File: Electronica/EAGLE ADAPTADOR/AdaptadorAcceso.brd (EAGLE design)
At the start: 160.5 x 111 mm, 9 parts

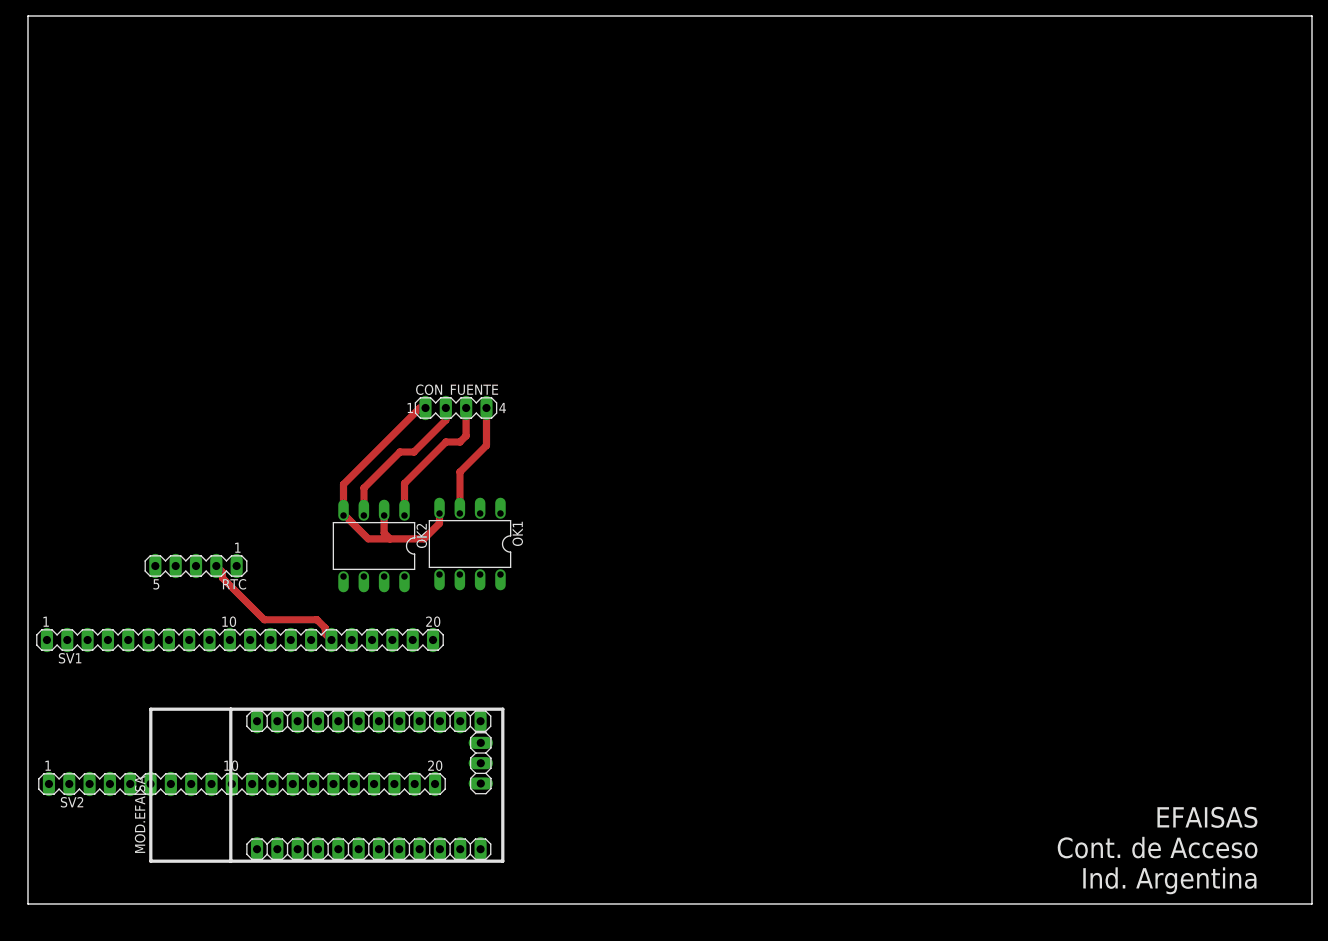
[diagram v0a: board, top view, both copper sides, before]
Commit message: PCB terminado - A revisar
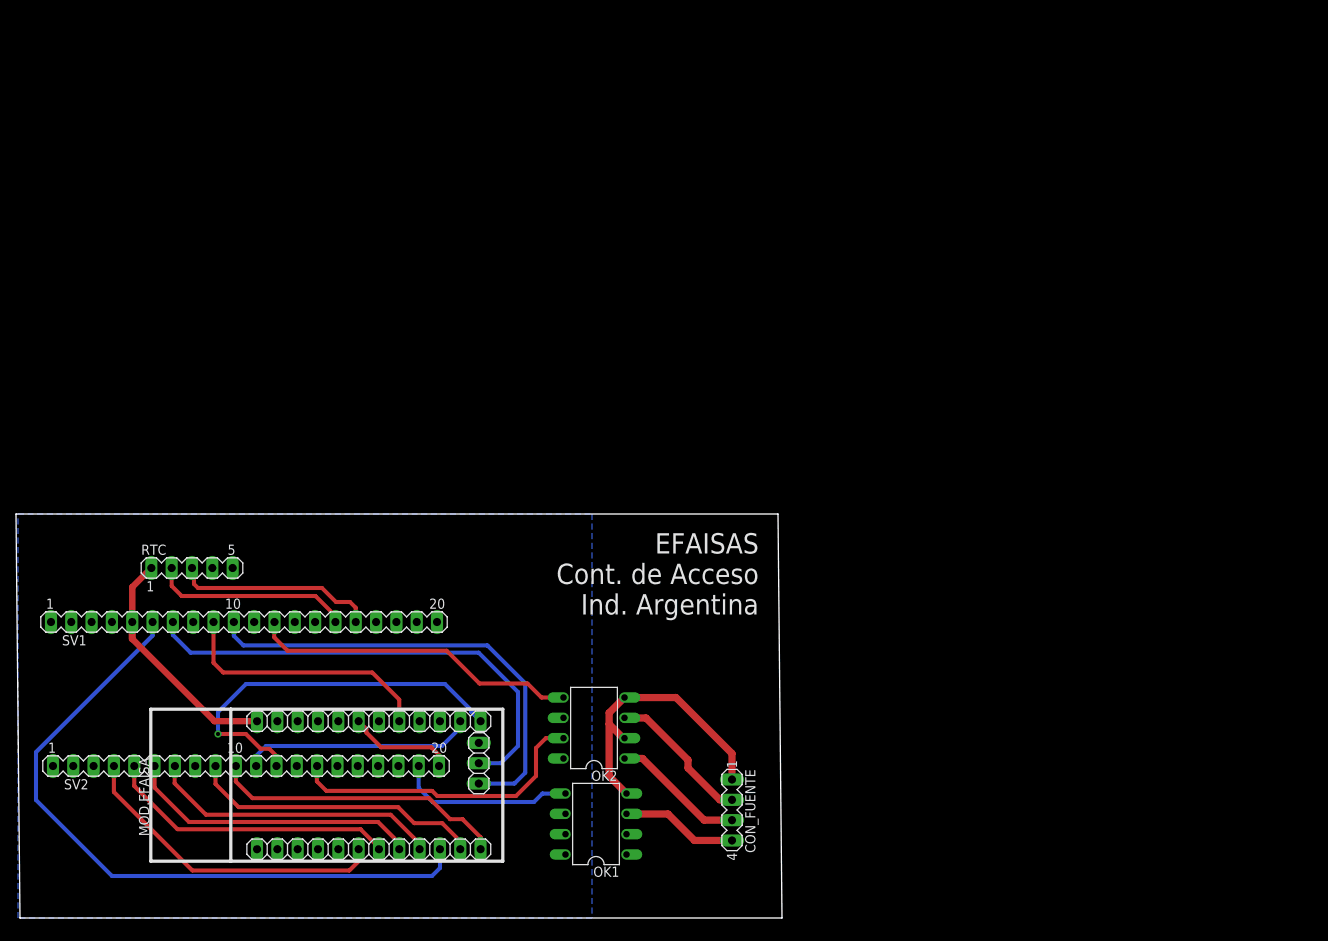
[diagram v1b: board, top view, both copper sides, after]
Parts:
- moved CON_FUENTE 61.0 mm to (88.0, 11.8), turned to 270 degrees
- moved OK1 38.4 mm to (71.0, 10.0), turned to 90 degrees
- moved OK2 35.7 mm to (70.8, 22.0), turned to 90 degrees
- moved SV1 2.30 mm to (27.0, 35.2)
- moved SV2 2.30 mm to (27.2, 17.2)
- moved RTC 0.56 mm to (20.5, 42.0), turned to 0 degrees
- moved J4 0.25 mm to (56.4, 17.6)
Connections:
- net N$4 renamed GND_FUENTE
- removed net GND_OPTO: OK1.6, OK2.6, OK2.8, SV2.3
- net GNDA: now also OK1.6, OK2.6, OK2.8, SV2.3
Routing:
- net IO21: track 0.00 -> 85.5 mm
- net IO17: track 0.00 -> 60.3 mm
- net IO18: track 0.00 -> 58.2 mm
- net IO39: track 0.00 -> 48.8 mm, vias 0 -> 1
- net C_OPTO3: track 0.00 -> 41.2 mm
- net IO48: track 0.00 -> 39.9 mm
- net C_OPTO2: track 0.00 -> 38.6 mm
- net IO41: track 0.00 -> 36.9 mm
- net IO46: track 0.00 -> 36.9 mm
- net IO42: track 0.00 -> 36.8 mm
- net IO45: track 0.00 -> 36.6 mm
- net IO47: track 0.00 -> 36.5 mm
- net IO16: track 0.00 -> 32.9 mm
- net +3V3: track 0.00 -> 29.7 mm
- net IO40: track 0.00 -> 29.1 mm
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- added copper zone on layer 16, net GNDA
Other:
- board size 160.5 x 111 mm -> 95.8 x 50.5 mm

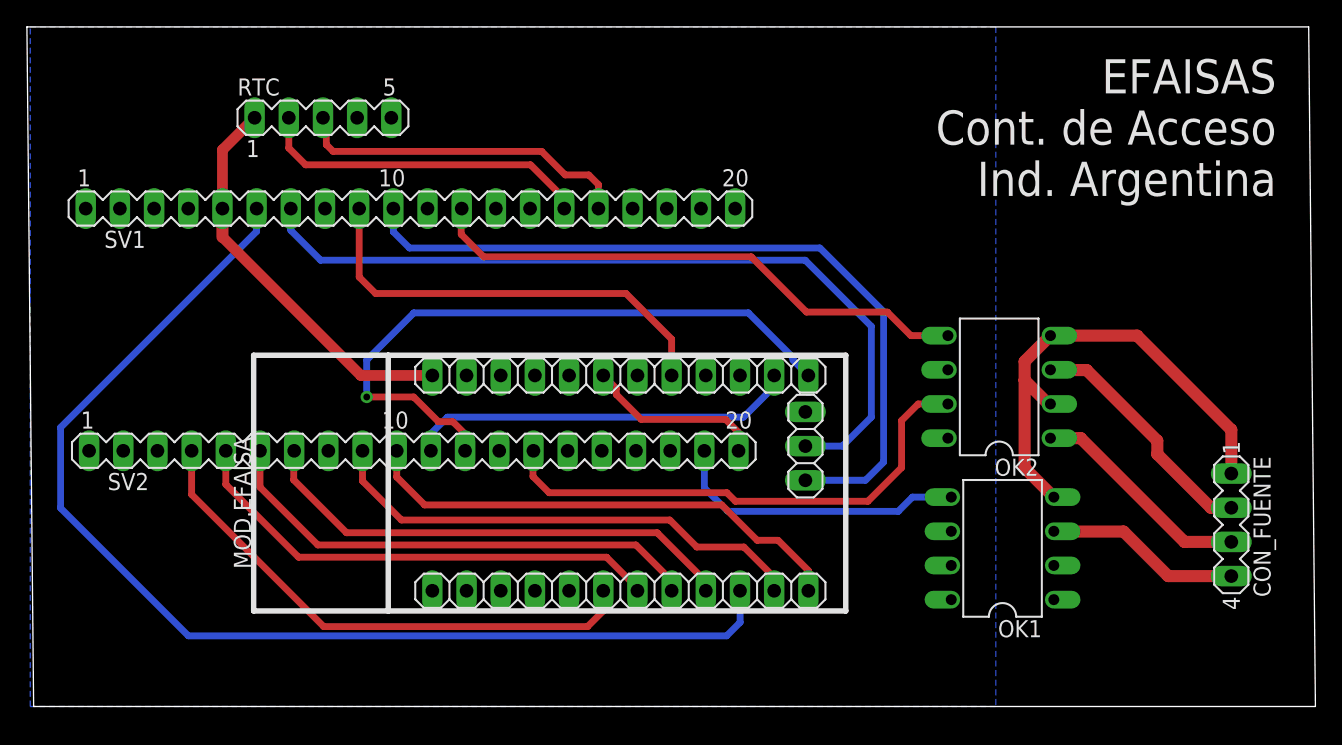
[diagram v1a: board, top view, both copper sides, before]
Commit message: Actualizacion PCB - A revisar
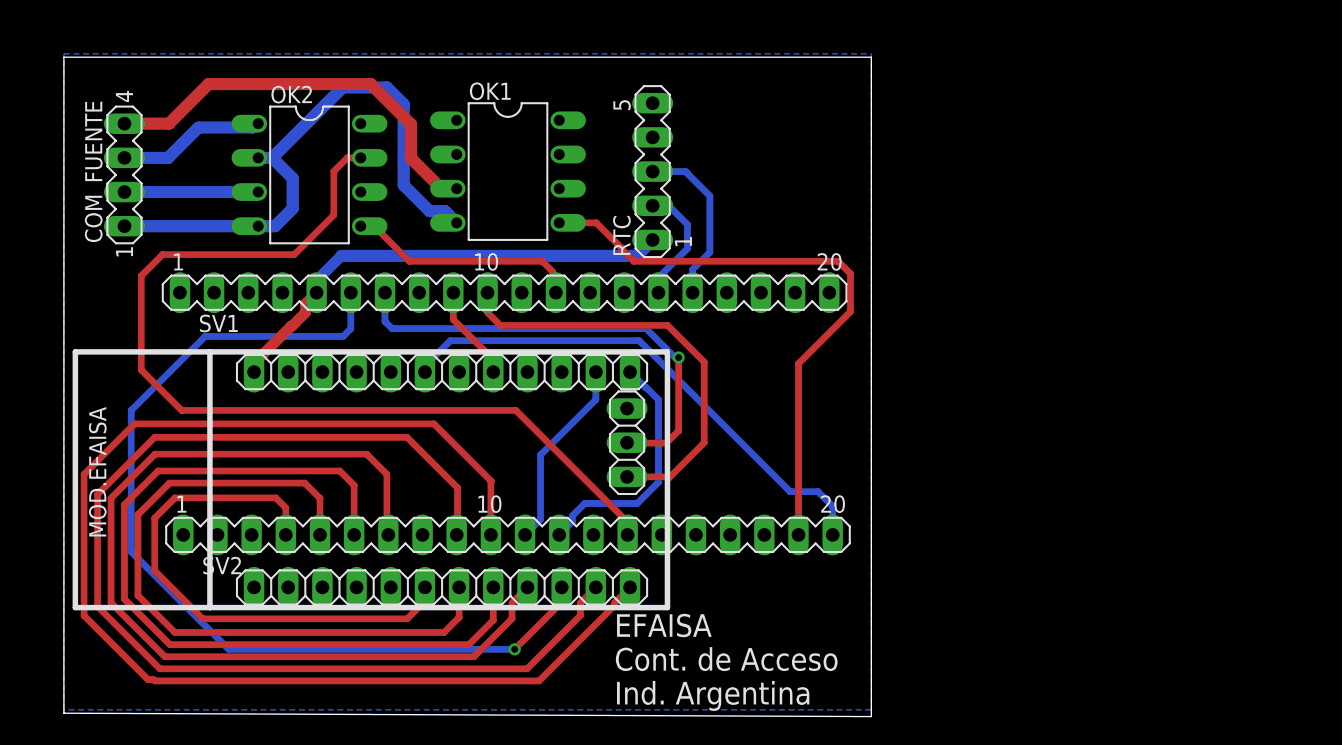
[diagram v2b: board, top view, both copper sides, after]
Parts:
- removed CON_FUENTE: (no value), con-lstb:MA04-1
- added COM_FUENTE: (no value), con-lstb:MA04-1
- moved OK2 53.6 mm to (19.5, 37.8), turned to 270 degrees
- moved OK1 46.2 mm to (34.2, 38.0), turned to 270 degrees
- moved RTC 24.8 mm to (45.0, 38.0), turned to 90 degrees
- moved J1 13.3 mm to (29.4, 23.1)
- moved J4 13.3 mm to (43.1, 17.9)
- moved MOD.EFAISA 13.3 mm to (29.4, 7.10)
- moved SV1 9.38 mm to (34.0, 29.0)
- moved SV2 9.38 mm to (34.2, 11.0)
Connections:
- net GND_FUENTE: now also COM_FUENTE.1; no longer CON_FUENTE.1
- net N$1: now also COM_FUENTE.4; no longer CON_FUENTE.4
- net N$2: now also COM_FUENTE.3; no longer CON_FUENTE.3
- net N$3: now also COM_FUENTE.2; no longer CON_FUENTE.2
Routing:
- net IO41: track 36.9 -> 93.6 mm
- net IO42: track 36.8 -> 83.9 mm
- net IO45: track 36.6 -> 70.2 mm
- net C_OPTO2: track 38.6 -> 70.6 mm
- net IO39: track 48.8 -> 18.3 mm, vias 1 -> 0
- net IO18: track 58.2 -> 31.9 mm
- net IO16: track 32.9 -> 7.13 mm
- net IO17: track 60.3 -> 34.7 mm, vias 0 -> 1
- net IO33: track 13.4 -> 38.7 mm
- net IO46: track 36.9 -> 61.3 mm
- net C_OPTO3: track 41.2 -> 17.3 mm
- net C_OPTO1: track 22.3 -> 44.3 mm
- net N$1: track 14.6 -> 30.6 mm
- net IO21: track 85.5 -> 69.6 mm, vias 0 -> 1
- net DATA_RTC: track 25.0 -> 9.12 mm
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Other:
- board size 95.8 x 50.5 mm -> 60 x 49 mm
- board text added: "EFAISA Cont. de Acceso Ind. Argentina"
- board text removed: "EFAISAS Cont. de Acceso Ind. Argentina"
